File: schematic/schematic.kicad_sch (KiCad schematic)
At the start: 34 parts

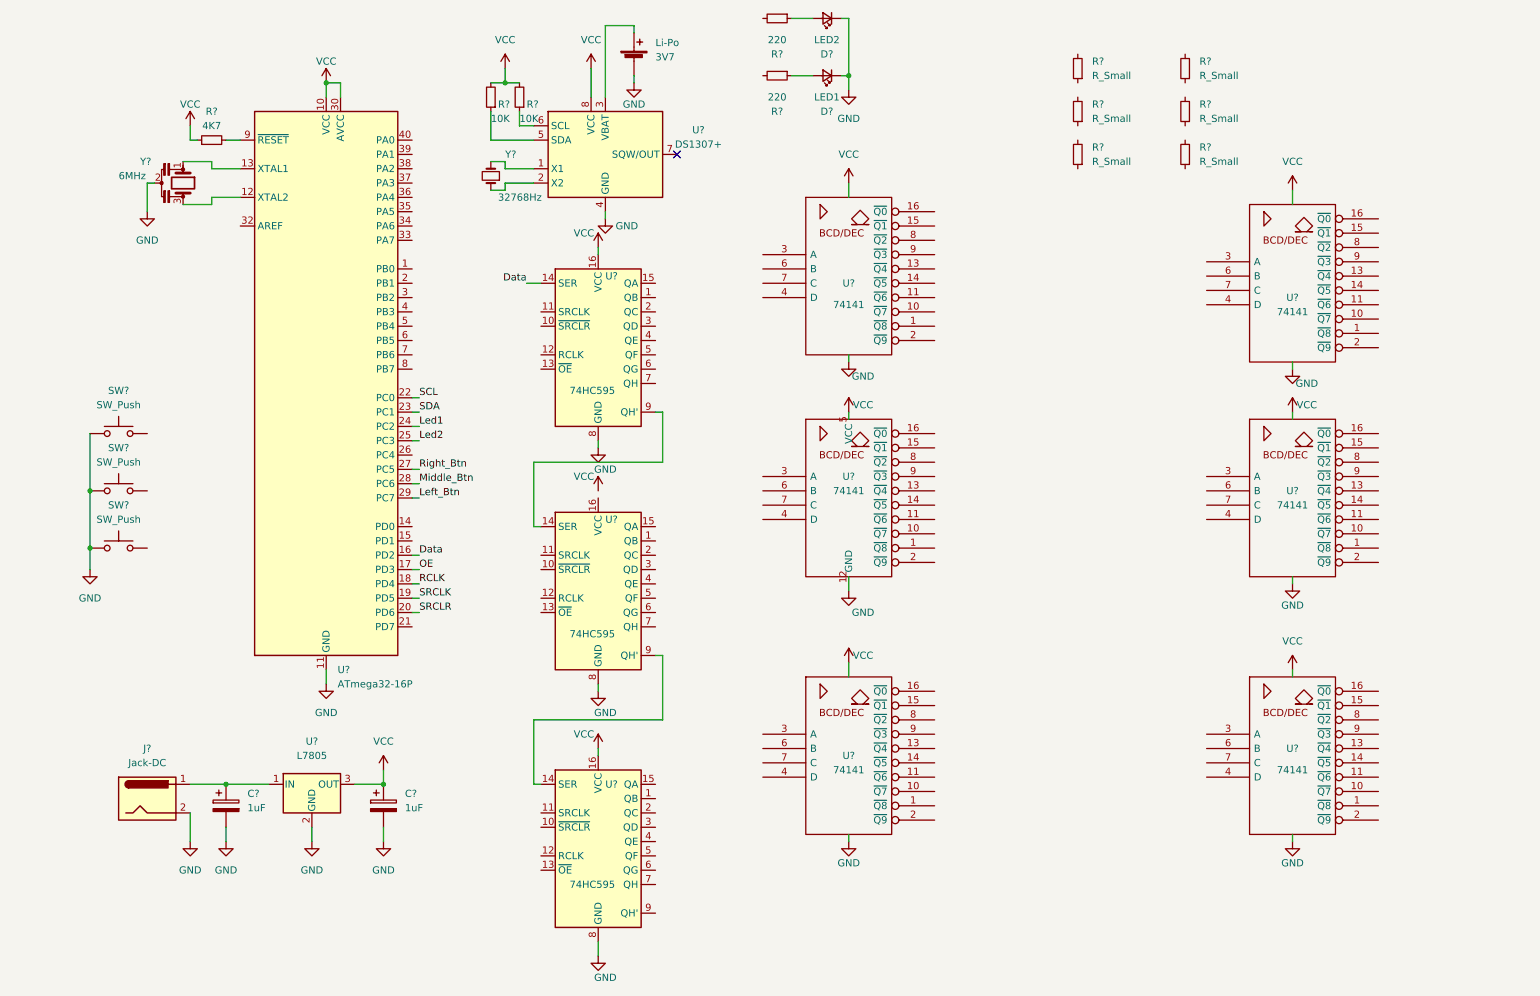
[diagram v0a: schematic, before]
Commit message: Schematic update
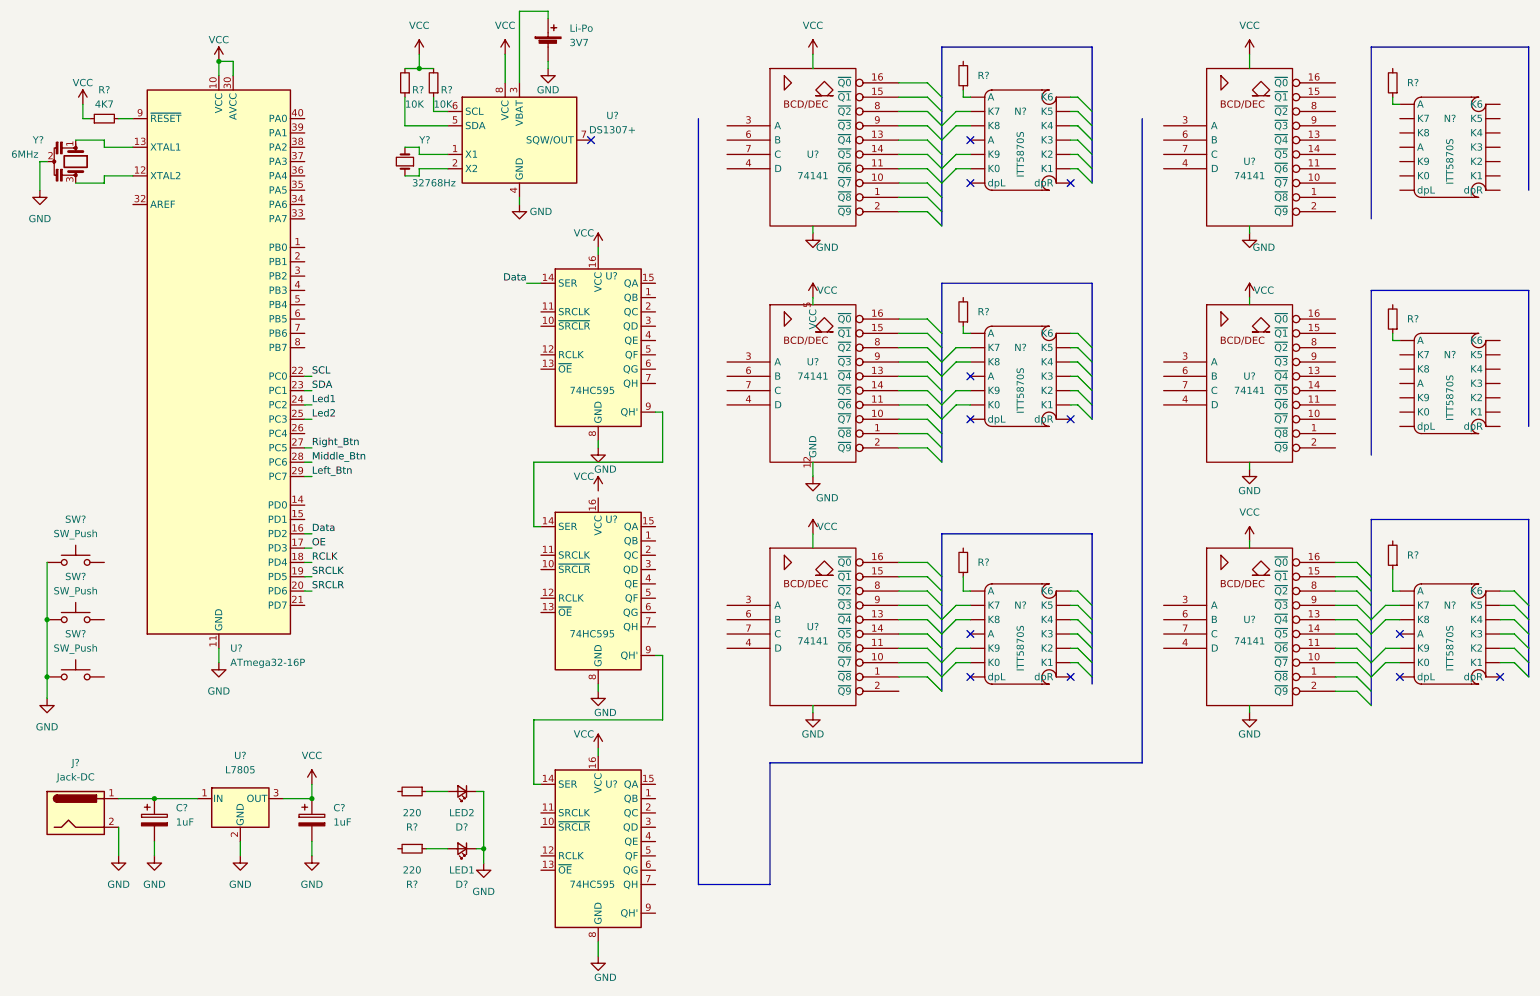
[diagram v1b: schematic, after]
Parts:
- removed R? (x5): R_Small, symbol Device:R_Small
- added N? (x6): ITT5870S, symbol ITT5870S:ITT5870S
- added R? (x5): R_Small, symbol Device:R_Small
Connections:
- net at R?.1: now also N?. (dpR)
- new net: N?. (dpR), R?.1 (x5)
- no-connect marks 1 -> 13
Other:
- moved on the sheet: C?, D?, J?, Li-Po, R?, SW?, U?, Y?

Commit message: Updated schematic
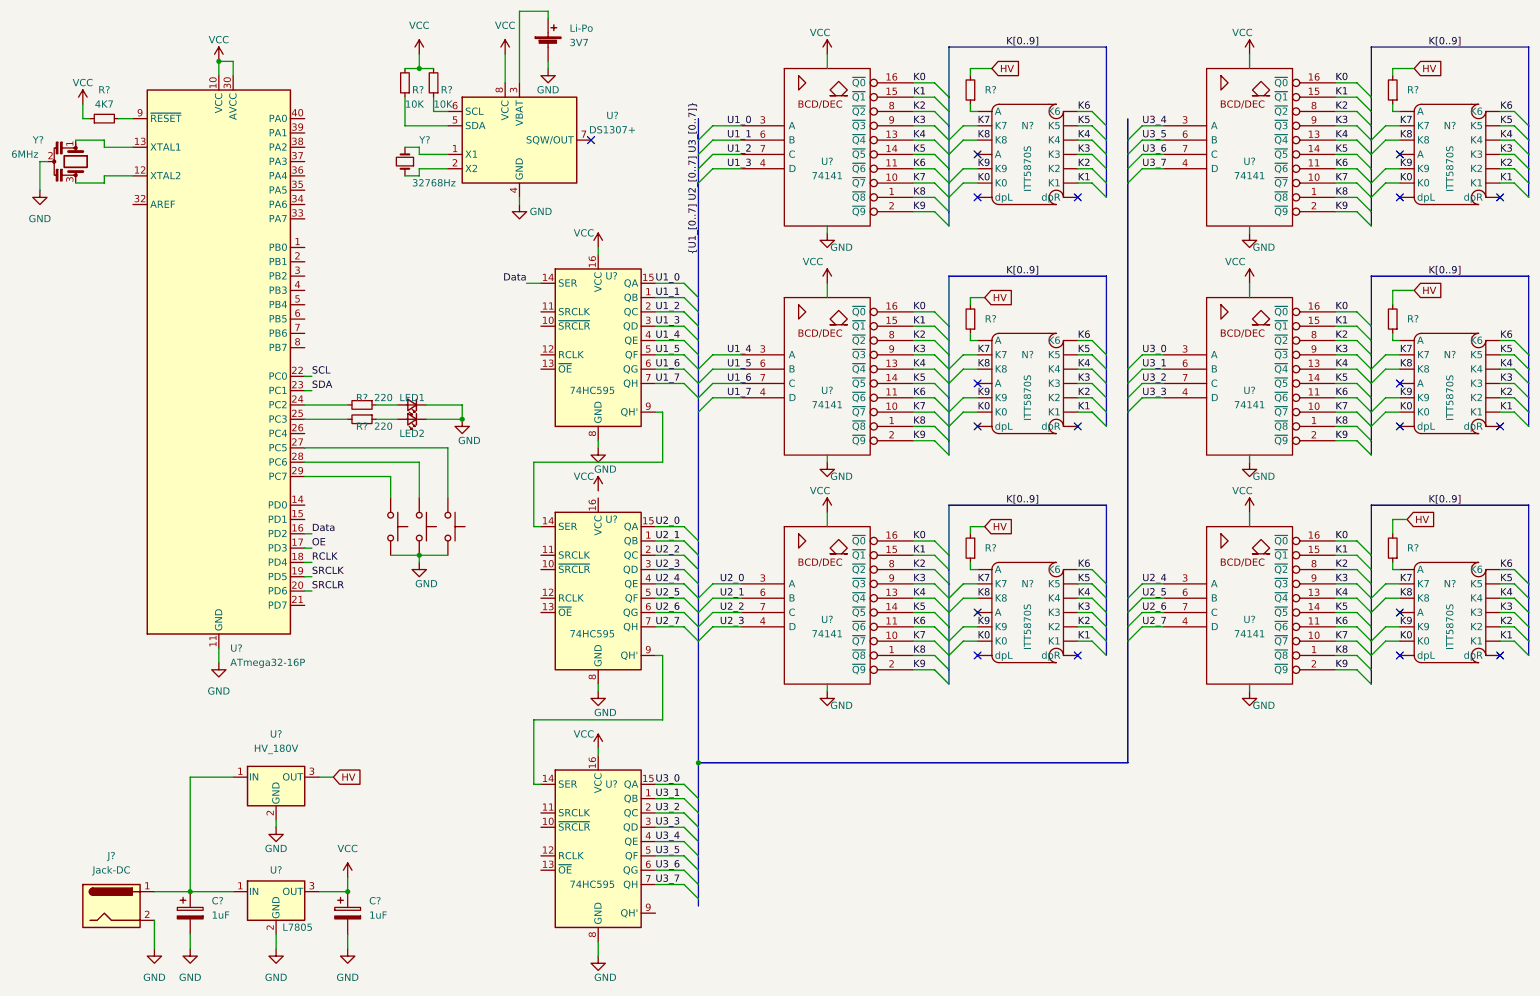
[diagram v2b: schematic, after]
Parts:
- removed N? (x5): ITT5870S, symbol ITT5870S:ITT5870S
- removed R? (x5): R_Small, symbol Device:R_Small
- removed SW? (x2): SW_Push, symbol Switch:SW_Push
- removed U? (x5): 74141, symbol 74xx_IEEE:74141
- added N? (x5): ITT5870S, symbol ITT5870S:ITT5870S
- added R? (x5): R_Small, symbol Device:R_Small
- added SW? (x2): SW_Push, symbol Switch:SW_Push
- added U?: HV_180V, symbol Regulator_Linear:L7805
- added U? (x5): 74141, symbol 74xx_IEEE:74141
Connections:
- net Led1 is gone; now on an unnamed net: U?.24 (PC2)
- net Led2 is gone; now on an unnamed net: U?.25 (PC3)
- net GND: now also SW?.2, SW?.2, SW?.2, U?.12 (GND), U?.12 (GND), U?.12 (GND), U?.12 (GND), U?.12 (GND), U?.2 (GND); no longer SW?.1
- net VCC: now also U?.5 (VCC), U?.5 (VCC), U?.5 (VCC), U?.5 (VCC), U?.5 (VCC)
- net at C?.1, J?.1, U?.1 (IN): now also U?.1 (IN)
- net K9: now reaches N?. (dpR)
- net K9: now also U?.2 (~{Q9}), N?. (dpR), N?. (dpR), N?. (dpR), N?. (dpR), N?. (dpR), U?.2 (~{Q9}), U?.2 (~{Q9}), U?.2 (~{Q9}), U?.2 (~{Q9}), U?.2 (~{Q9})
- net U1_1: now reaches U?.1 (QB)
- net U1_1: now also U?.6 (B)
- net U1_0: now reaches U?.15 (QA)
- net U1_0: now also U?.3 (A)
- net U1_2: now reaches U?.2 (QC)
- net U1_2: now also U?.7 (C)
- net U1_3: now reaches U?.3 (QD)
- net U1_3: now also U?.4 (D)
- net U1_4: now reaches U?.4 (QE)
- net U1_4: now also U?.3 (A)
- net U1_5: now reaches U?.5 (QF)
- net U1_5: now also U?.6 (B)
- net U1_6: now reaches U?.6 (QG)
- net U1_6: now also U?.7 (C)
- net U1_7: now reaches U?.7 (QH)
- net U1_7: now also U?.4 (D)
- net HV: now reaches R?.2
- net HV: now also R?.2, R?.2, R?.2, R?.2, R?.2, U?.3 (OUT)
- net U3_1: now reaches U?.1 (QB)
- net U3_1: now also U?.6 (B)
- net U3_0: now reaches U?.15 (QA)
- net U3_0: now also U?.3 (A)
- net U3_2: now reaches U?.2 (QC)
- net U3_2: now also U?.7 (C)
- net U3_3: now reaches U?.3 (QD)
- net U3_3: now also U?.4 (D)
- net U3_4: now reaches U?.4 (QE)
- net U3_4: now also U?.3 (A)
- net U3_5: now reaches U?.5 (QF)
- net U3_5: now also U?.6 (B)
- net U3_6: now reaches U?.6 (QG)
- net U3_6: now also U?.7 (C)
- net U3_7: now reaches U?.7 (QH)
- net U3_7: now also U?.4 (D)
- net U2_1: now reaches U?.1 (QB)
- net U2_1: now also U?.6 (B)
- net U2_0: now reaches U?.15 (QA)
- net U2_0: now also U?.3 (A)
- net U2_2: now reaches U?.2 (QC)
- net U2_2: now also U?.7 (C)
- net U2_3: now reaches U?.3 (QD)
- net U2_3: now also U?.4 (D)
- net U2_4: now reaches U?.4 (QE)
- net U2_4: now also U?.3 (A)
- net U2_5: now reaches U?.5 (QF)
- net U2_5: now also U?.6 (B)
- net U2_6: now reaches U?.6 (QG)
- net U2_6: now also U?.7 (C)
- net U2_7: now reaches U?.7 (QH)
- net U2_7: now also U?.4 (D)
- net K8: now reaches U?.1 (~{Q8})
- net K8: now also N?. (dpR), N?. (dpR), N?. (dpR), N?. (dpR), N?. (dpR), N?. (dpR), U?.1 (~{Q8}), U?.1 (~{Q8}), U?.1 (~{Q8}), U?.1 (~{Q8}), U?.1 (~{Q8})
- net K7: now reaches U?.10 (~{Q7})
- net K7: now also N?. (dpR), N?. (dpR), N?. (dpR), N?. (dpR), N?. (dpR), N?. (dpR), U?.10 (~{Q7}), U?.10 (~{Q7}), U?.10 (~{Q7}), U?.10 (~{Q7}), U?.10 (~{Q7})
- net K6: now reaches U?.11 (~{Q6})
- net K6: now also N?. (dpR), N?. (dpR), N?. (dpR), N?. (dpR), N?. (dpR), N?. (dpR), U?.11 (~{Q6}), U?.11 (~{Q6}), U?.11 (~{Q6}), U?.11 (~{Q6}), U?.11 (~{Q6})
- net K4: now reaches U?.13 (~{Q4})
- net K4: now also N?. (dpR), N?. (dpR), N?. (dpR), N?. (dpR), N?. (dpR), N?. (dpR), U?.13 (~{Q4}), U?.13 (~{Q4}), U?.13 (~{Q4}), U?.13 (~{Q4}), U?.13 (~{Q4})
- net K5: now reaches U?.14 (~{Q5})
- net K5: now also N?. (dpR), N?. (dpR), N?. (dpR), N?. (dpR), N?. (dpR), N?. (dpR), U?.14 (~{Q5}), U?.14 (~{Q5}), U?.14 (~{Q5}), U?.14 (~{Q5}), U?.14 (~{Q5})
- net K1: now reaches U?.15 (~{Q1})
- net K1: now also N?. (dpR), N?. (dpR), N?. (dpR), N?. (dpR), N?. (dpR), N?. (dpR), U?.15 (~{Q1}), U?.15 (~{Q1}), U?.15 (~{Q1}), U?.15 (~{Q1}), U?.15 (~{Q1})
- net K0: now reaches U?.16 (~{Q0})
- net K0: now also N?. (dpR), N?. (dpR), N?. (dpR), N?. (dpR), N?. (dpR), N?. (dpR), U?.16 (~{Q0}), U?.16 (~{Q0}), U?.16 (~{Q0}), U?.16 (~{Q0}), U?.16 (~{Q0})
- net K2: now reaches U?.8 (~{Q2})
- net K2: now also N?. (dpR), N?. (dpR), N?. (dpR), N?. (dpR), N?. (dpR), N?. (dpR), U?.8 (~{Q2}), U?.8 (~{Q2}), U?.8 (~{Q2}), U?.8 (~{Q2}), U?.8 (~{Q2})
- net K3: now reaches U?.9 (~{Q3})
- net K3: now also N?. (dpR), N?. (dpR), N?. (dpR), N?. (dpR), N?. (dpR), N?. (dpR), U?.9 (~{Q3}), U?.9 (~{Q3}), U?.9 (~{Q3}), U?.9 (~{Q3}), U?.9 (~{Q3})
- net Left_Btn: no longer names the net of U?.29 (PC7)
- net Left_Btn: now also SW?.1
- net Middle_Btn: no longer names the net of U?.28 (PC6)
- net Middle_Btn: now also SW?.1
- net Right_Btn: no longer names the net of U?.27 (PC5)
- net Right_Btn: now also SW?.1
- new net: N?. (dpR), R?.1 (x5)
- no-connect marks 13 -> 19
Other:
- moved on the sheet: C?, J?, N?, R?, U?
